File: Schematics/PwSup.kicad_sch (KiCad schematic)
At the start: 37 parts, among them J3 Neutral, J4 Px N, J5 PXB10C, J6 Phase, J7 Px Ph, SW2 SW_SPST, U1 TL072, U4 LM317_TO-220, U5 LM337_TO220

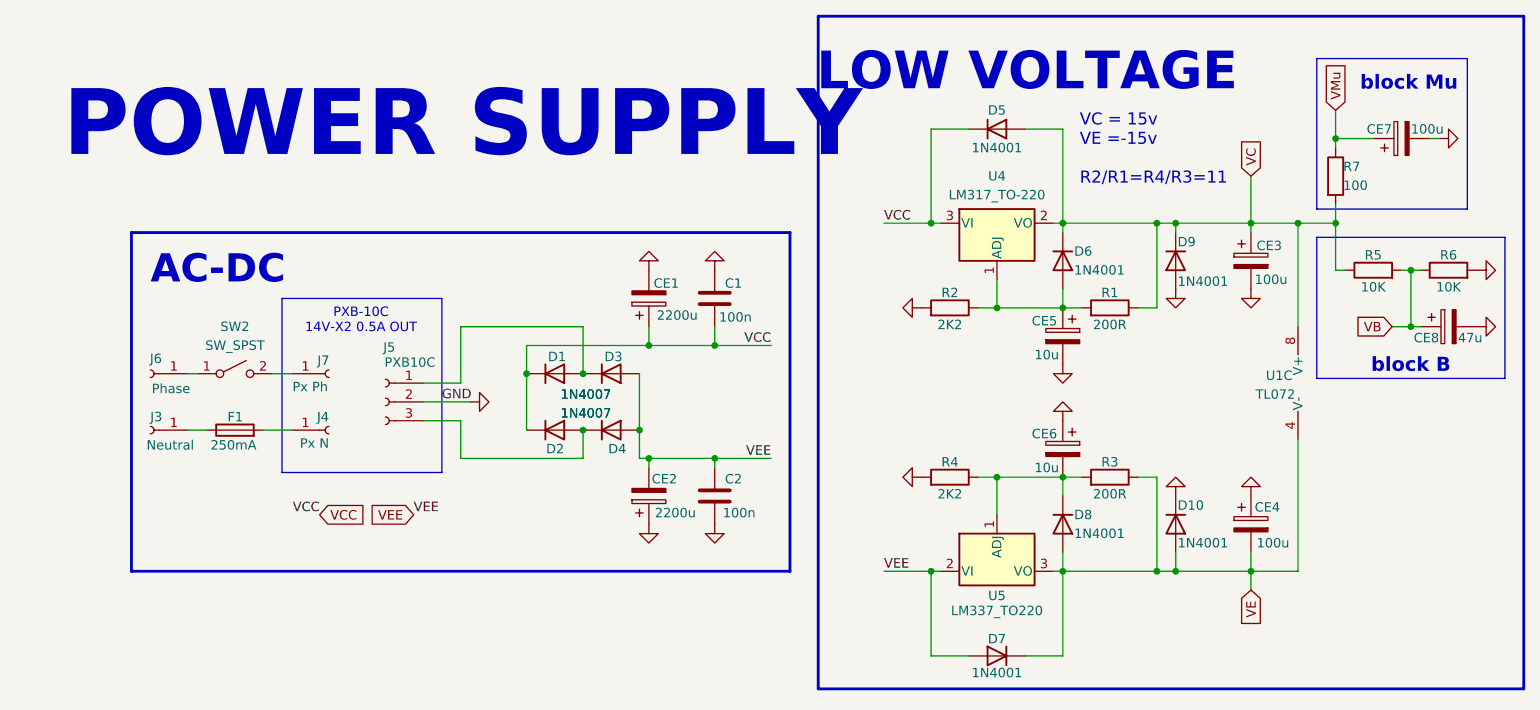
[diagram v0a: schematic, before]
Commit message: Cosmetic upd
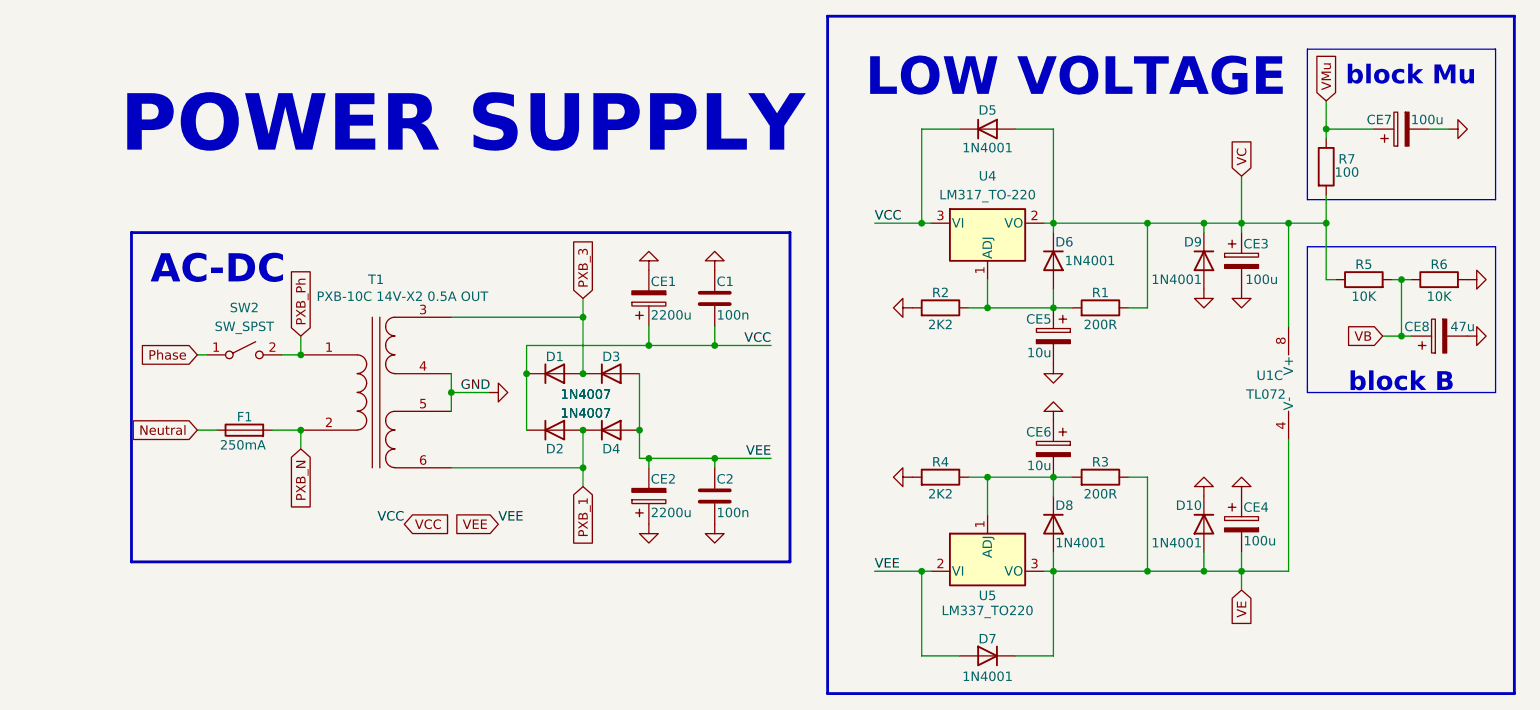
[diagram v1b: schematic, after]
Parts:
- removed J3: Neutral, PrLib:connector, symbol Connector:Conn_01x01_Socket
- removed J4: Px N, PrLib:connector, symbol Connector:Conn_01x01_Socket
- removed J5: PXB10C, Connector_JST:JST_XH_B3B-XH-A_1x03_P2.50mm_Vertical, symbol Connector:Conn_01x03_Socket
- removed J6: Phase, symbol Connector:Conn_01x01_Socket
- removed J7: Px Ph, symbol Connector:Conn_01x01_Socket
- added T1: PXB-10C 14V-X2 0.5A OUT, symbol Device:Transformer_1P_2S
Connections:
- net GND: now also T1.4 (SB), T1.5 (SC)
- net PXB_N: now reaches F1.2
- net PXB_N: now also T1.2 (AB)
- net Phase: now reaches SW2.1 (A)
- net PXB_3: now reaches D1.2 (A), D3.1 (K)
- net PXB_3: now also T1.3 (SA)
- net PXB_1: now reaches D2.2 (A), D4.1 (K)
- net PXB_1: now also T1.6 (SD)
- net PXB_Ph: now reaches SW2.2 (B)
- net PXB_Ph: now also T1.1 (AA)
- net Neutral: now reaches F1.1
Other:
- note removed: "PXB-10C 14V-X2 0.5A OUT"
- note removed: "VC = 15v VE =-15v R2/R1=R4/R3=11"
- moved on the sheet: CE3, CE4, CE5, CE6, CE7, CE8, D10, D5, D6, D7, D8, D9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
